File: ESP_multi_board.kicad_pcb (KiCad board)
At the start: 2 copper layers, 36 parts, among them IC101 L298, P101 CONN_01X02, P102 CONN_01X06, P103 CONN_01X02, P104 CONN_01X06, P105 CONN_01X06, P106 CONN_01X03, P107 CONN_I2C_MPU6050, P108 CONN_PINES_DIG, P109 CONN_01X04, SW101 SW_PUSH_SMALL, SW102 SWITCH_INV, U1 LD1117S33TR, U102 ESP-12, U103 MAX11605EEE+, U104 MCP23008

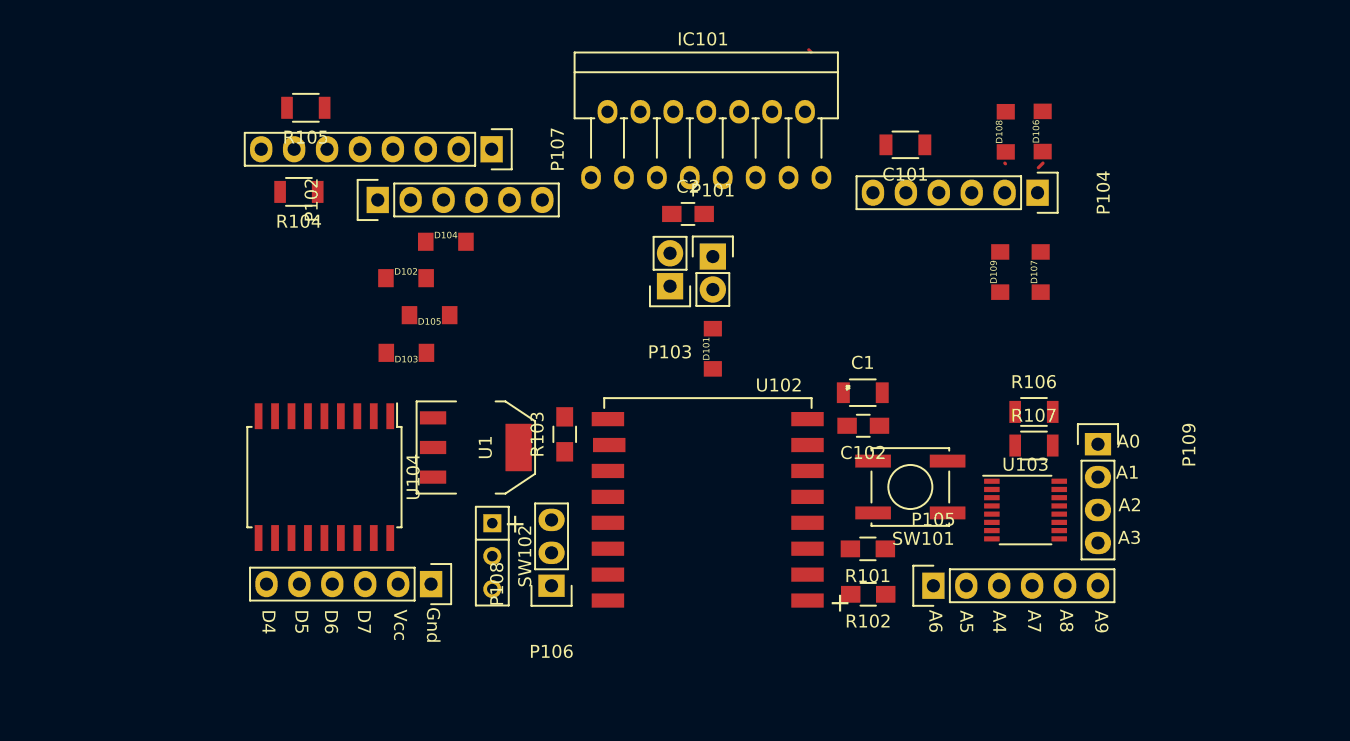
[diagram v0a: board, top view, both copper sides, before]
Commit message: placa actualizada
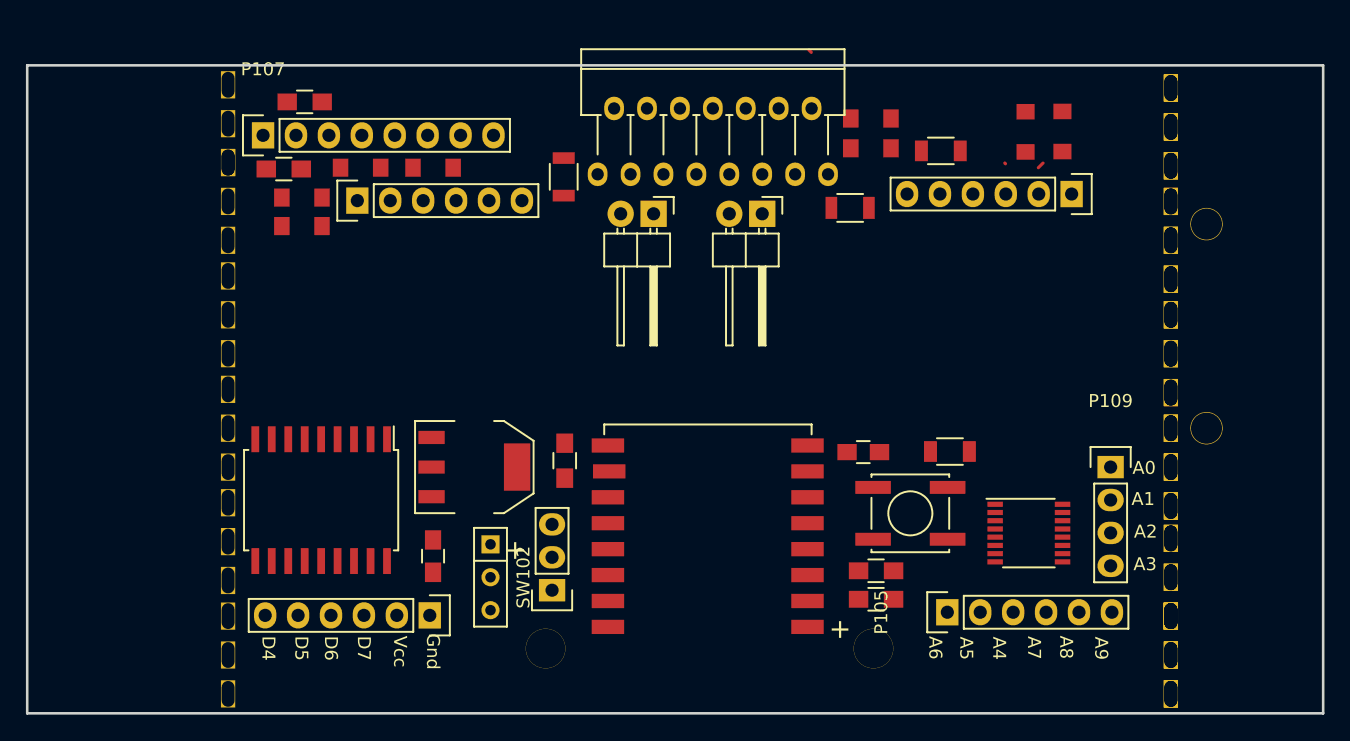
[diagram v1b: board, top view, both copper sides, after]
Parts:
- removed D101: D, diodos_smd:SMD_D_SMA-Sub-2
- added REF**: troquel, taladros:troquel_3, F.Cu at (99.5, 69.5)
- added REF** (x2): troquel, taladros:troquel_3, F.Cu at (172.2, 87.2)
- added REF** (x2): troquel, taladros:troquel_3, F.Cu at (172.2, 78.5)
- added REF** (x2): troquel, taladros:troquel_3, F.Cu at (172.2, 69.8)
- added REF** (x2): troquel, taladros:troquel_3, F.Cu at (172.2, 110.5)
- added REF** (x2): troquel, taladros:troquel_3, F.Cu at (172.2, 104.5)
- added REF**: 1pin, Connect:1pin, F.Cu at (175.0, 93.0)
- added REF**: 1pin, Connect:1pin, F.Cu at (175.0, 77.2)
- added REF**: troquel, taladros:troquel_3, F.Cu at (99.5, 75.5)
- added REF**: 1pin, Connect:1pin, F.Cu at (149.3, 110.0)
- added REF**: 1pin, Connect:1pin, F.Cu at (124.0, 110.0)
- added REF** (x2): troquel, taladros:troquel_3, F.Cu at (172.2, 96.0)
- added REF**: troquel, taladros:troquel_3, F.Cu at (99.5, 84.2)
- added REF**: troquel, taladros:troquel_3, F.Cu at (99.5, 93.0)
- added REF**: troquel, taladros:troquel_3, F.Cu at (99.5, 101.8)
- added REF**: troquel, taladros:troquel_3, F.Cu at (99.5, 110.5)
- P101, P103: footprint Pin_Headers:Pin_Header_Straight_1x02 -> Pin_Headers:Pin_Header_Angled_1x02
- P105: footprint Socket_Strips:Socket_Strip_Straight_1x06 -> Pin_Headers:Pin_Header_Straight_1x06
- P107: footprint Pin_Headers:Pin_Header_Straight_1x08 -> Socket_Strips:Socket_Strip_Straight_1x08
- P109: footprint Socket_Strips:Socket_Strip_Straight_1x04 -> Pin_Headers:Pin_Header_Straight_1x04
- R104, R105: value 47k -> 4.7k; footprint Resistors_SMD:R_1206 -> Resistors_SMD:R_0805_HandSoldering
- moved R106 40.6 mm to (125.4, 73.6), turned to 90 degrees
- moved C2 32.9 mm to (115.3, 102.9), turned to 270 degrees
- moved R107 23.2 mm to (147.5, 76.0)
- moved P107 17.7 mm to (102.2, 70.4), turned to 0 degrees
- moved D107 17.7 mm to (149.1, 69.1), turned to 0 degrees
- moved D103 14.7 mm to (109.7, 72.9)
- moved D109 13.8 mm to (149.1, 71.4), turned to 0 degrees
- moved D105 13.4 mm to (105.2, 75.2), turned to 180 degrees
- moved D102 8.98 mm to (105.2, 77.4), turned to 0 degrees
- moved C1 8.11 mm to (155.2, 94.8), turned to 180 degrees
- moved D104 5.80 mm to (115.3, 72.9)
- moved P103 5.73 mm to (132.3, 76.5), turned to 270 degrees
- moved P101 5.04 mm to (140.7, 76.5), turned to 270 degrees
- moved C101 2.77 mm to (154.5, 71.6)
- moved P104 2.63 mm to (164.6, 74.9)
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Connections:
- P101 pad 2: Net-(D101-Pad1) -> Net-(P101-Pad2)
- SW102 pad 2: Net-(D101-Pad2) -> Net-(P101-Pad2)
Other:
- board outline added: 100 x 50 mm
